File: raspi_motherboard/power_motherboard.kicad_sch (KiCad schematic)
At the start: 19 parts, among them J1 GPIO, J2 Conn_02x04_Top_Bottom

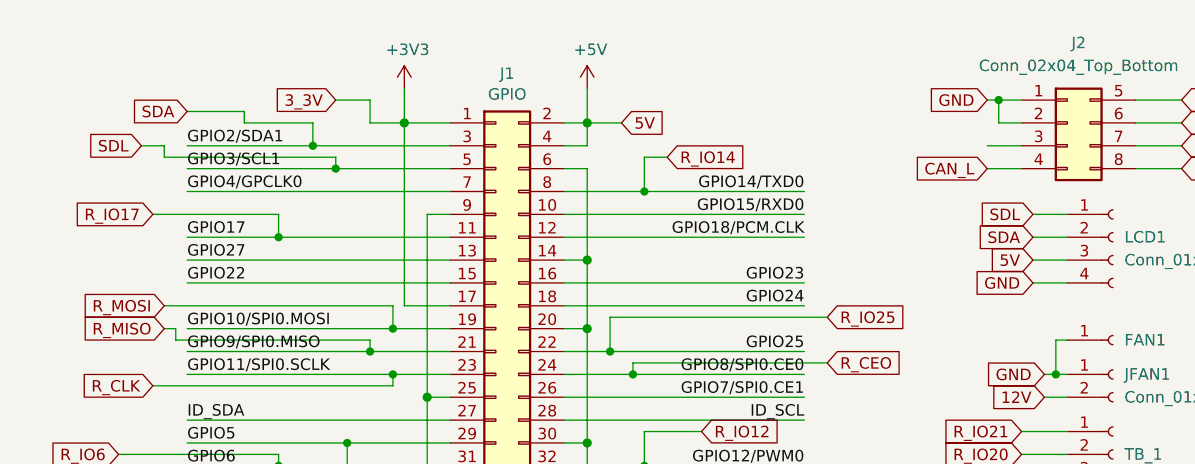
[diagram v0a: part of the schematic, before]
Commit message: Production version
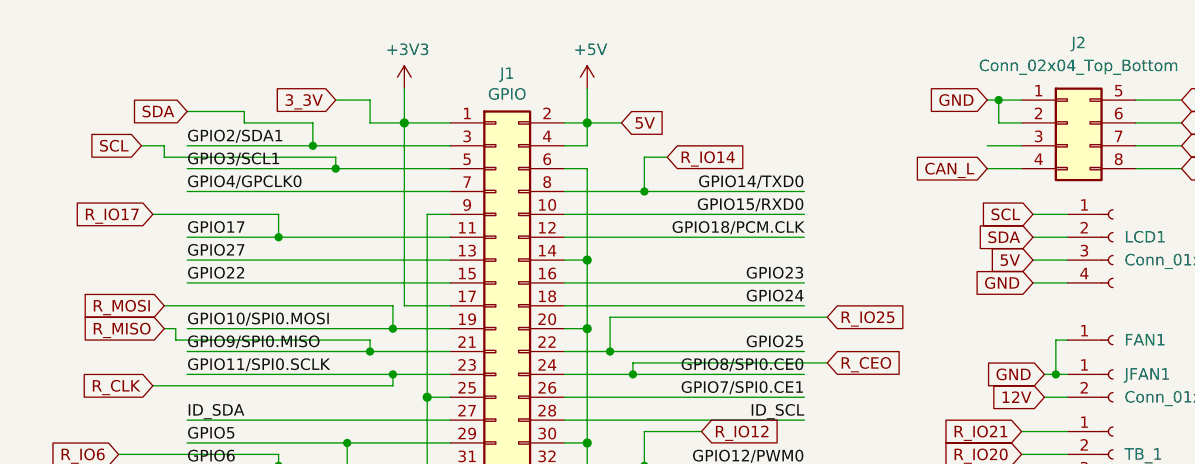
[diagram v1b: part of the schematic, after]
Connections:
- net SDL renamed SCL
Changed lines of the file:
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@@
 		)
 	)
-	(global_label "SDL"
+	(global_label "SCL"
 		(shape input)
 		(at 26.67 30.48 180)
@@
 		)
 	)
-	(global_label "SDL"
+	(global_label "SCL"
 		(shape input)
 		(at 125.73 38.1 180)
